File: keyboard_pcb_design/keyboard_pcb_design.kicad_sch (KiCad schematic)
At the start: 45 parts, among them J1 Conn_01x03, J2 USB4105-GF-A, SW1 Switch, SW2 Switch, SW3 Switch, SW4 Switch, SW5 Switch, SW6 PTS645SH50SMTR92LFS, SW7 PTS645SH50SMTR92LFS, U1 SC09147, U2 NCP1117-3.3_SOT223, U3 MX25L3233FM2I-08Q, U4 SMF05CT1G, X1 ABM8-272-T3

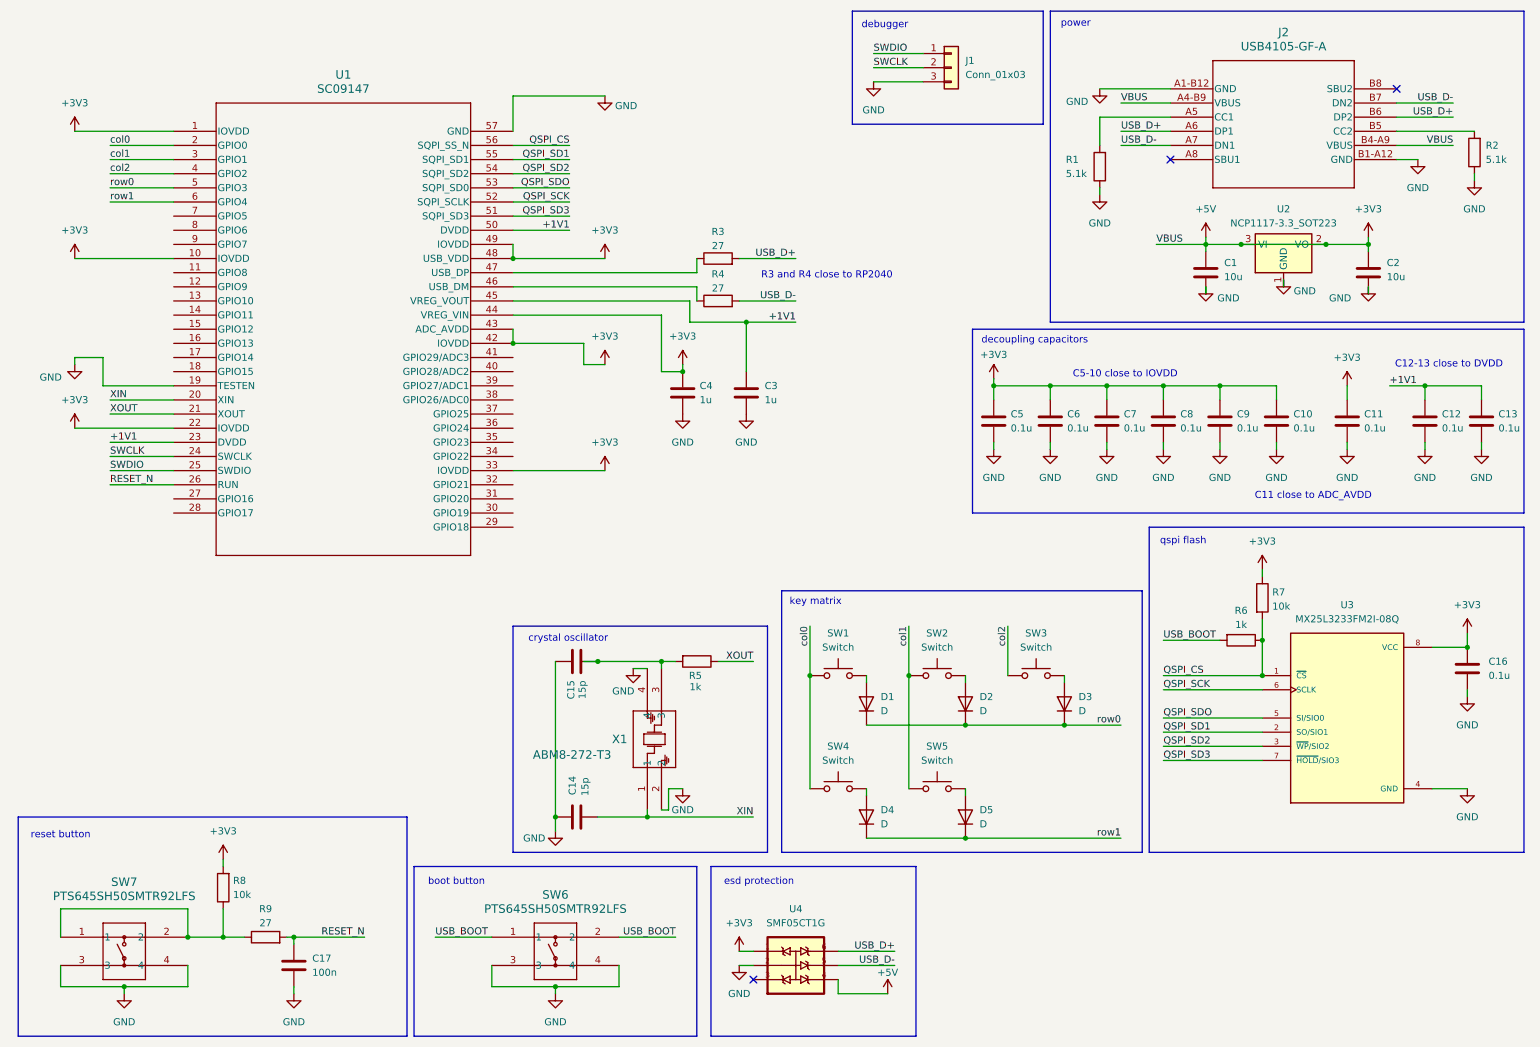
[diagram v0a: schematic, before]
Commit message: complete joystick schematic
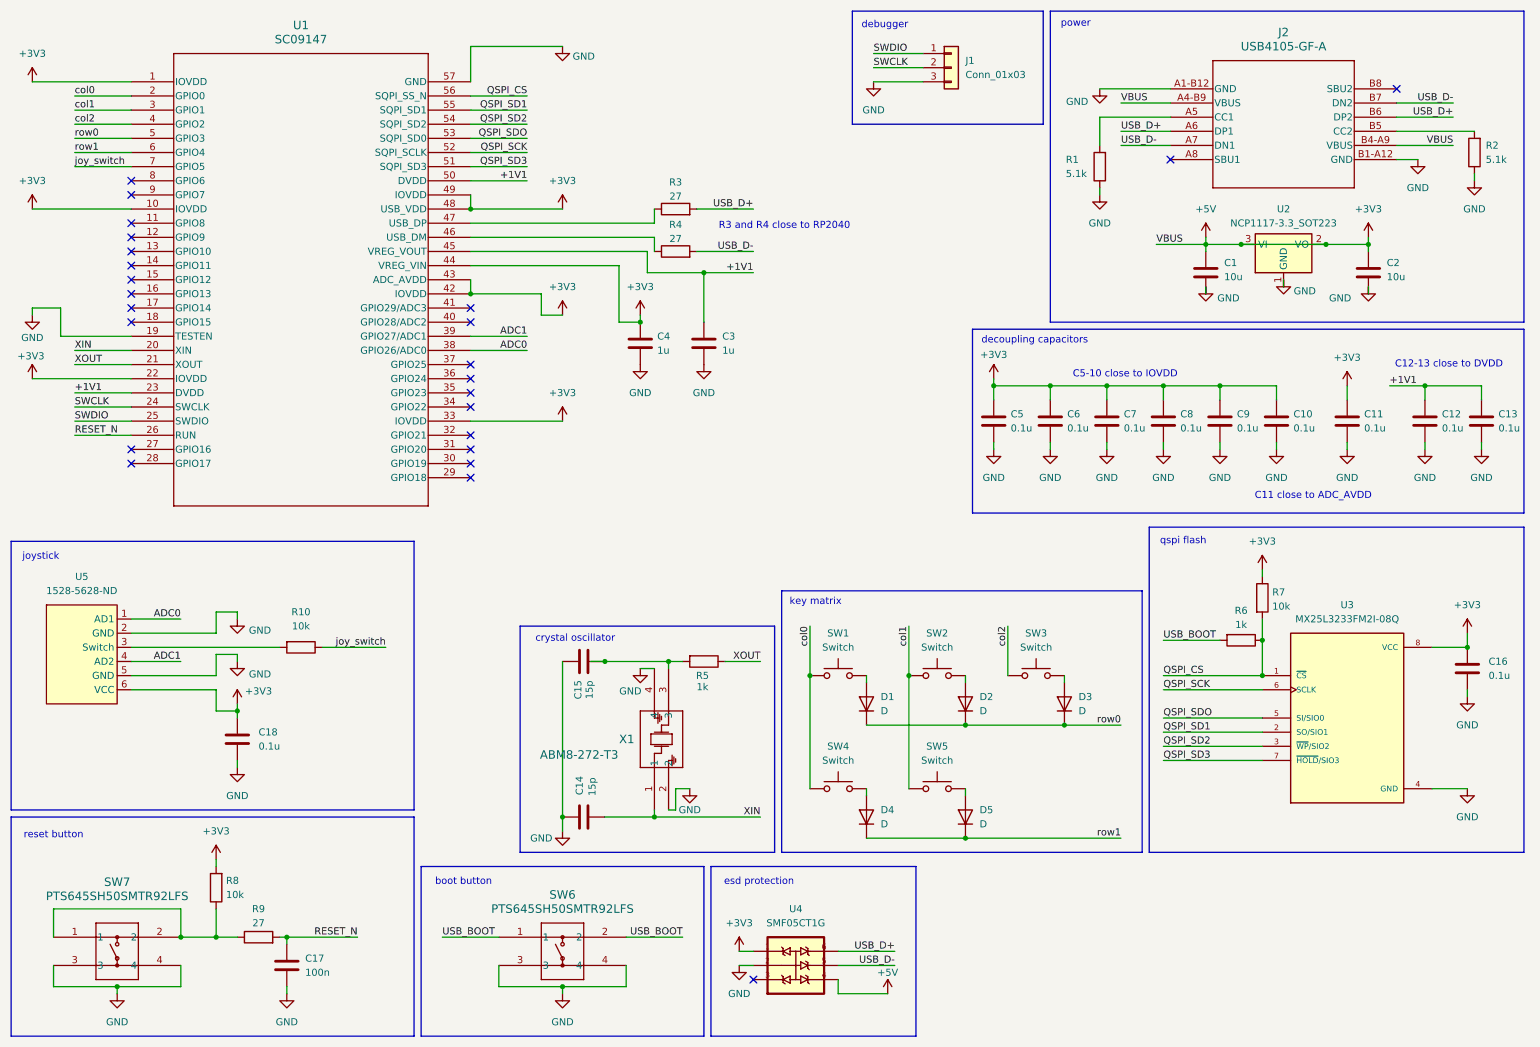
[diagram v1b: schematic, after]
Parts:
- added C18: 0.1u, Capacitor_SMD:C_0201_0603Metric, symbol Device:C
- added R10: 10k, symbol Device:R
- added U5: 1528-5628-ND, symbol keyboard_library:1528-5628-ND
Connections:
- net +3V3: now also C18.1, U5.6 (VCC)
- net GND: now also C18.2, U5.2 (GND), U5.5 (GND)
- net ADC0: now reaches U1.38 (GPIO26/ADC0)
- net ADC0: now also U5.1 (AD1)
- net ADC1: now reaches U1.39 (GPIO27/ADC1)
- net ADC1: now also U5.4 (AD2)
- net joy_switch: now reaches U1.7 (GPIO5)
- net joy_switch: now also R10.1
- new net: R10.2, U5.3 (Switch)
- no-connect marks 3 -> 25
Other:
- note added: "joystick"
- moved on the sheet: C14, C15, C17, C3, C4, R3, R4, R5, R8, R9, SW6, SW7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
